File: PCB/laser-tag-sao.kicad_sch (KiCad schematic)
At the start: 20 parts, among them J1 SAO Connector, Q1 PN2222A, SW1 SW_Push, SW2 SW_Push, SW3 SW_Push, U1 ATtiny84-20P, U2 TSOP38438, U3 OLED_0.91_128x32

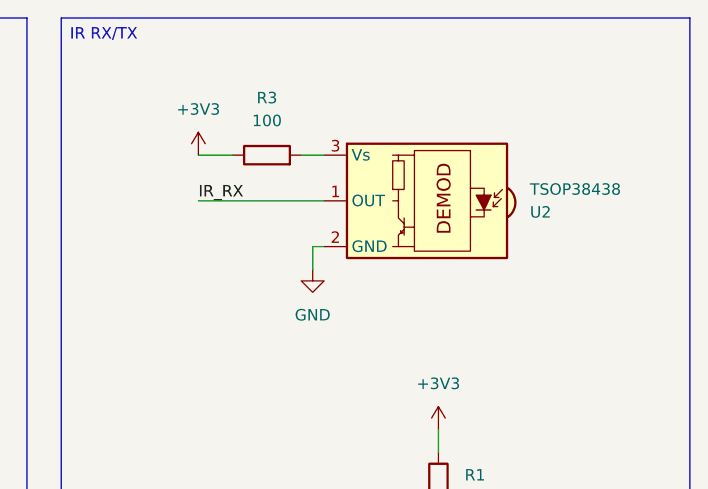
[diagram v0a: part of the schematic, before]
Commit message: updating again
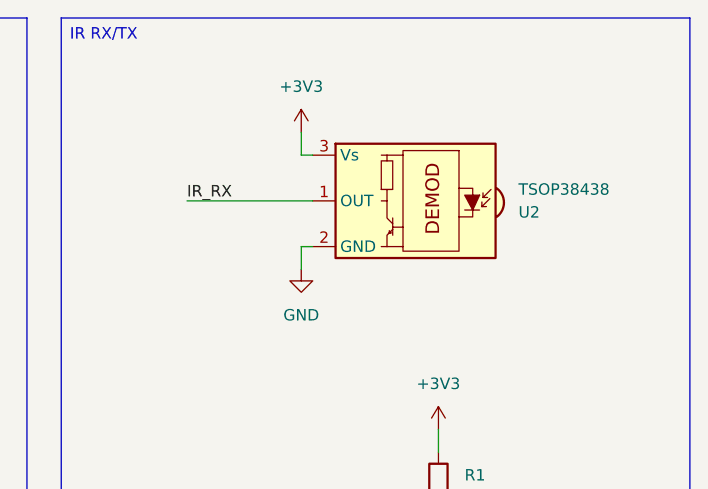
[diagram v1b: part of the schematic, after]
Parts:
- removed R3: 100, symbol Device:R
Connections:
- net +3V3: now also U2.3 (Vs)
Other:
- moved on the sheet: U2
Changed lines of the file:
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@@
-	(wire
-		(pts
-			(xy 223.52 33.02) (xy 227.33 33.02)
-		)
-		(stroke
-			(width 0)
-			(type default)
-		)
-	)
 	(wire
 		(pts
@@
 	(wire
 		(pts
-			(xy 223.52 38.1) (xy 237.49 38.1)
+			(xy 222.25 38.1) (xy 236.22 38.1)
 		)
 		(stroke
@@
 	(wire
 		(pts
+			(xy 234.95 30.48) (xy 234.95 33.02)
+		)
+		(stroke
+			(width 0)
+			(type default)
+		)
+	)
+	(wire
+		(pts
 			(xy 157.48 46.99) (xy 144.78 46.99)
 		)
@@
 	(wire
 		(pts
-			(xy 236.22 43.18) (xy 236.22 45.72)
+			(xy 234.95 43.18) (xy 234.95 45.72)
 		)
 		(stroke
@@
 	(wire
 		(pts
+			(xy 234.95 33.02) (xy 236.22 33.02)
+		)
+		(stroke
+			(width 0)
+			(type default)
+		)
+	)
+	(wire
+		(pts
 			(xy 30.48 41.91) (xy 44.45 41.91)
 		)
@@
 	(wire
 		(pts
-			(xy 237.49 43.18) (xy 236.22 43.18)
+			(xy 236.22 43.18) (xy 234.95 43.18)
 		)
 		(stroke
@@
 		(pts
 			(xy 167.64 74.93) (xy 144.78 74.93)
-		)
-		(stroke
-			(width 0)
-			(type default)
-		)
-	)
-	(wire
-		(pts
-			(xy 234.95 33.02) (xy 237.49 33.02)
 		)
 		(stroke
@@
 	)
 	(label "IR_RX"
-		(at 223.52 38.1 0)
+		(at 222.25 38.1 0)
 		(effects
 			(font
@@
 	(symbol
 		(lib_id "power:+3V3")
-		(at 223.52 33.02 0)
+		(at 234.95 30.48 0)
 		(unit 1)
 		(body_style 1)
@@
 		(fields_autoplaced yes)
 		(property "Reference" "#PWR017"
-			(at 223.52 36.83 0)
+			(at 234.95 34.29 0)
 			(hide yes)
 			(show_name no)
@@
 		)
 		(property "Value" "+3V3"
-			(at 223.52 27.94 0)
+			(at 234.95 25.4 0)
 			(show_name no)
 			(do_not_autoplace no)
@@
 		)
 		(property "Footprint" ""
-			(at 223.52 33.02 0)
+			(at 234.95 30.48 0)
 			(hide yes)
 			(show_name no)
@@
 		)
 		(property "Datasheet" ""
-			(at 223.52 33.02 0)
+			(at 234.95 30.48 0)
 			(hide yes)
 			(show_name no)
@@
 		)
 		(property "Description" "Power symbol creates a global label with name \"+3V3\""
-			(at 223.52 33.02 0)
+			(at 234.95 30.48 0)
 			(hide yes)
 			(show_name no)
@@
 				(path "/bd497134-ab55-4d01-915d-3710c30e2e14"
 					(reference "#PWR017")
-					(unit 1)
-				)
-			)
-		)
-	)
-	(symbol
-		(lib_id "Device:R")
-		(at 231.14 33.02 90)
-		(unit 1)
-		(body_style 1)
-		(exclude_from_sim no)
-		(in_bom yes)
-		(on_board yes)
-		(in_pos_files yes)
-		(dnp no)
-		(fields_autoplaced yes)
-		(property "Reference" "R3"
-			(at 231.14 26.67 90)
-			(show_name no)
-			(do_not_autoplace no)
-			(effects
-				(font
-					(size 1.27 1.27)
-				)
-			)
-		)
-		(property "Value" "100"
-			(at 231.14 29.21 90)
-			(show_name no)
-			(do_not_autoplace no)
-			(effects
-				(font
-					(size 1.27 1.27)
-				)
-			)
-		)
-		(property "Footprint" ""
-			(at 231.14 34.798 90)
-			(hide yes)
-			(show_name no)
-			(do_not_autoplace no)
-			(effects
-				(font
-					(size 1.27 1.27)
-				)
-			)
-		)
-		(property "Datasheet" ""
-			(at 231.14 33.02 0)
-			(hide yes)
-			(show_name no)
-			(do_not_autoplace no)
-			(effects
-				(font
-					(size 1.27 1.27)
-				)
-			)
-		)
-		(property "Description" "Resistor"
-			(at 231.14 33.02 0)
-			(hide yes)
-			(show_name no)
-			(do_not_autoplace no)
-			(effects
-				(font
-					(size 1.27 1.27)
-				)
-			)
-		)
-		(pin "2"
-		)
-		(pin "1"
-		)
-		(instances
-			(project "laser-tag-sao"
-				(path "/bd497134-ab55-4d01-915d-3710c30e2e14"
-					(reference "R3")
 					(unit 1)
 				)
@@
 	(symbol
 		(lib_id "Interface_Optical:TSOP384xx")
-		(at 247.65 38.1 0)
+		(at 246.38 38.1 0)
 		(mirror y)
 		(unit 1)
@@
 		(dnp no)
 		(property "Reference" "U2"
-			(at 260.35 39.3701 0)
+			(at 259.08 39.3701 0)
 			(show_name no)
 			(do_not_autoplace no)
@@
 		)
 		(property "Value" "TSOP38438"
-			(at 260.35 36.8301 0)
+			(at 259.08 36.8301 0)
 			(show_name no)
 			(do_not_autoplace no)
@@
 		)
 		(property "Footprint" "OptoDevice:Vishay_MINICAST-3Pin"
-			(at 248.92 47.625 0)
+			(at 247.65 47.625 0)
 			(hide yes)
 			(show_name no)
@@
 		)
 		(property "Datasheet" "http://www.vishay.com/docs/82491/tsop382.pdf"
-			(at 231.14 30.48 0)
+			(at 229.87 30.48 0)
 			(hide yes)
 			(show_name no)
@@
 		)
 		(property "Description" "Photo Modules for PCM Remote Control Systems"
-			(at 247.65 38.1 0)
+			(at 246.38 38.1 0)
 			(hide yes)
 			(show_name no)
@@
 	(symbol
 		(lib_id "power:GND")
-		(at 236.22 45.72 0)
+		(at 234.95 45.72 0)
 		(unit 1)
 		(body_style 1)
@@
 		(fields_autoplaced yes)
 		(property "Reference" "#PWR07"
-			(at 236.22 52.07 0)
+			(at 234.95 52.07 0)
 			(hide yes)
 			(show_name no)
@@
 		)
 		(property "Value" "GND"
-			(at 236.22 50.8 0)
+			(at 234.95 50.8 0)
 			(show_name no)
 			(do_not_autoplace no)
@@
 		)
 		(property "Footprint" ""
-			(at 236.22 45.72 0)
+			(at 234.95 45.72 0)
 			(hide yes)
 			(show_name no)
@@
 		)
 		(property "Datasheet" ""
-			(at 236.22 45.72 0)
+			(at 234.95 45.72 0)
 			(hide yes)
 			(show_name no)
@@
 		)
 		(property "Description" "Power symbol creates a global label with name \"GND\" , ground"
-			(at 236.22 45.72 0)
-			(hide yes)
-			(show_name no)
+			(at 234.95 45.72 0)
+			(hide yes)
+			(show_name no)
